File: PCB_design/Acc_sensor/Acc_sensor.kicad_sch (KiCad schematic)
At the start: 41 parts, among them Q1 NMOS, Q2 NMOS, SW1 SW_SPST, U1 ESP32-C3, U2 LIS2DE12, U3 DW01A, U3 MAX17263xxTE, U4 TLV75509PDBV, U5 TPS22917LDBV, U6 TLV75533PDBV

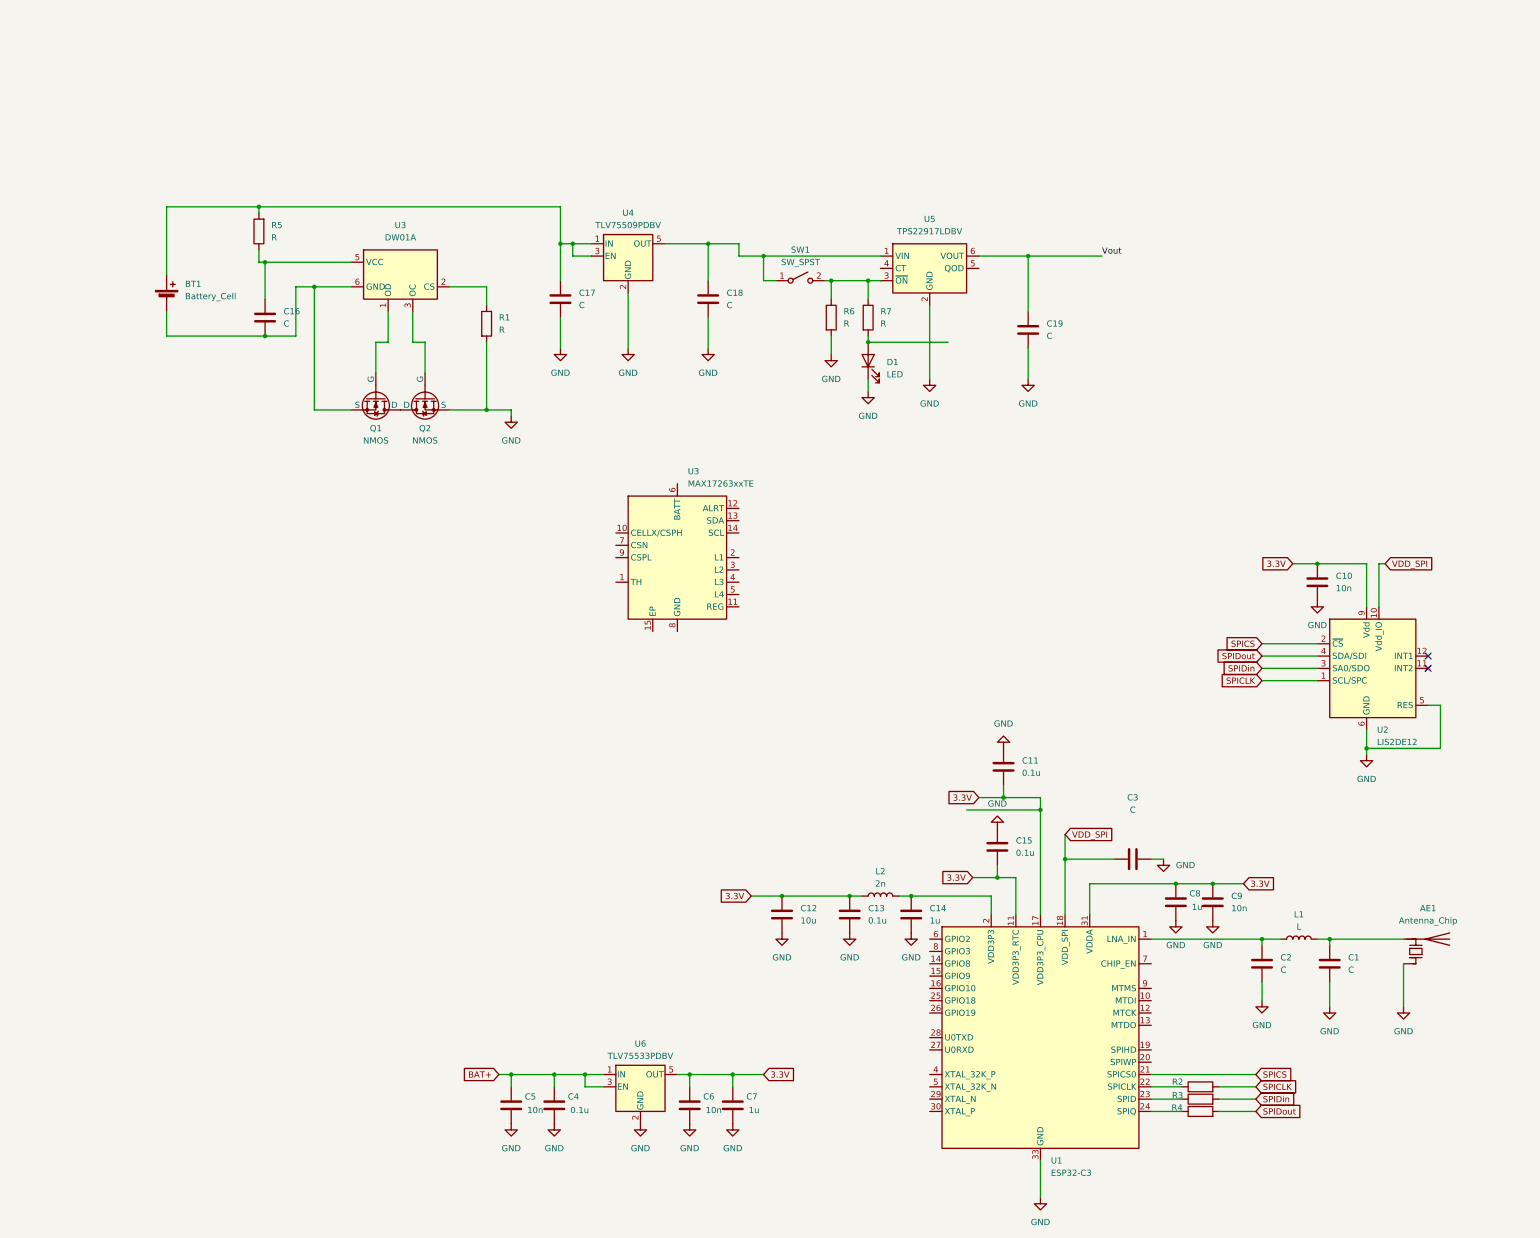
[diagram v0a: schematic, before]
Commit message: update
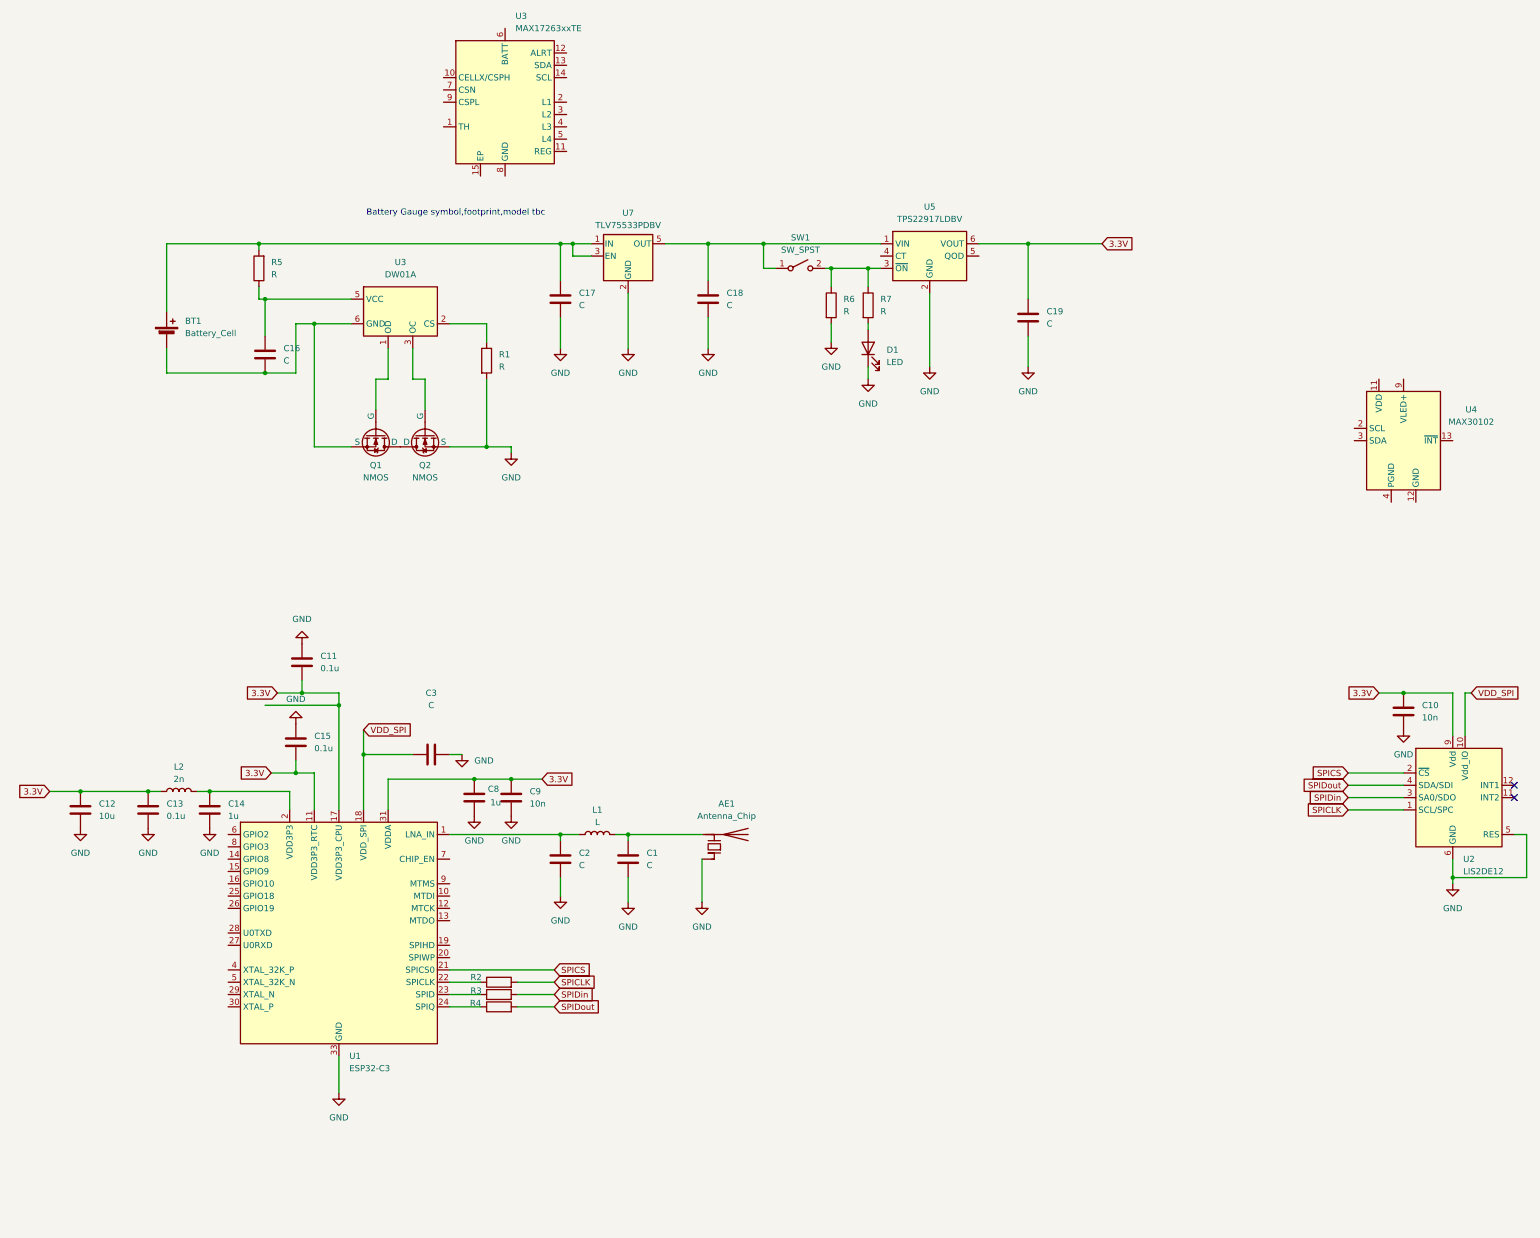
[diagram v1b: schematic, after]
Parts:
- removed C4: 0.1u, symbol Device:C
- removed C5, C6: 10n, symbol Device:C
- removed C7: 1u, symbol Device:C
- removed U4: TLV75509PDBV, Package_TO_SOT_SMD:SOT-23-5, symbol Regulator_Linear:TLV75509PDBV
- removed U6: TLV75533PDBV, Package_TO_SOT_SMD:SOT-23-5, symbol Regulator_Linear:TLV75533PDBV
- added U4: MAX30102, OptoDevice:Maxim_OLGA-14_3.3x5.6mm_P0.8mm, symbol Sensor:MAX30102
- added U7: TLV75533PDBV, Package_TO_SOT_SMD:SOT-23-5, symbol Regulator_Linear:TLV75533PDBV
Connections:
- net Vout is gone; now on net 3.3V: C19.1, U5.6 (VOUT)
- net GND: now also U7.2 (GND)
- net at C18.1, SW1.1 (A), U5.1 (VIN): now also U7.5 (OUT)
- net at BT1.1 (+), C17.1, R5.2: now also U7.1 (IN), U7.3 (EN)
- new net: U4.10 (VLED+), U4.9 (VLED+)
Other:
- note added: "Battery Gauge symbol,footprint,model tbc"
- moved on the sheet: AE1, BT1, C1, C10, C11, C12, C13, C14, C15, C16, C19, C2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
